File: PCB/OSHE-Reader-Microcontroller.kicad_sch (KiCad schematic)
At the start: 1 part

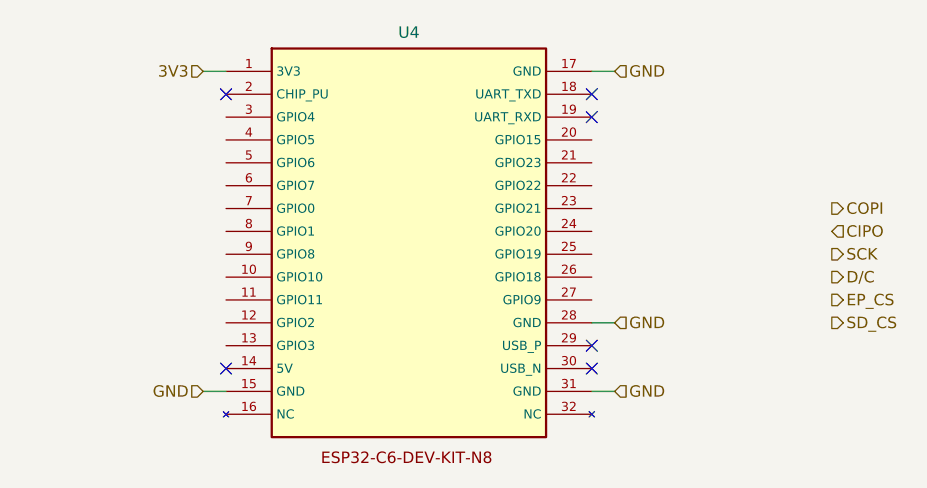
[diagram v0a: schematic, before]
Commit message: HOPEFULLY GOOD FOR EVER (good for first semester) :)
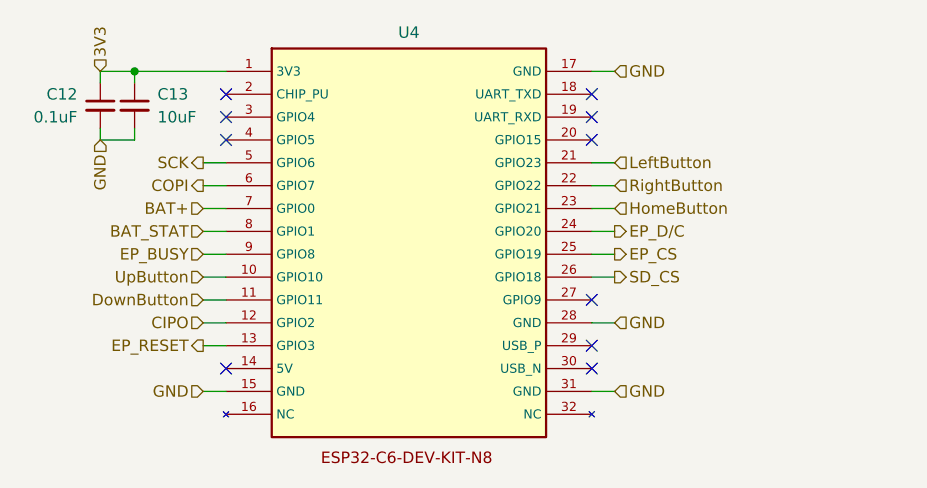
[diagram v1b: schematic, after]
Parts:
- added C12: 0.1uF, symbol Device:C_Small
- added C13: 10uF, symbol Device:C_Small
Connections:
- net 3V3: now also C12.1, C13.1
- net CIPO: now also U4.12 (GPIO2)
- net COPI: now also U4.6 (GPIO7)
- net EP_CS: now also U4.25 (GPIO19)
- net GND: now also C12.2, C13.2
- net SCK: now also U4.5 (GPIO6)
- net SD_CS: now also U4.26 (GPIO18)
- net UpButton: now reaches U4.10 (GPIO10)
- net DownButton: now reaches U4.11 (GPIO11)
- net EP_RESET: now reaches U4.13 (GPIO3)
- net LeftButton: now reaches U4.21 (GPIO23)
- net RightButton: now reaches U4.22 (GPIO22)
- net HomeButton: now reaches U4.23 (GPIO21)
- net EP_D/C: now reaches U4.24 (GPIO20)
- net BAT+: now reaches U4.7 (GPIO0)
- net BAT_STAT: now reaches U4.8 (GPIO1)
- net EP_BUSY: now reaches U4.9 (GPIO8)
- no-connect marks 6 -> 10

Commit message: small
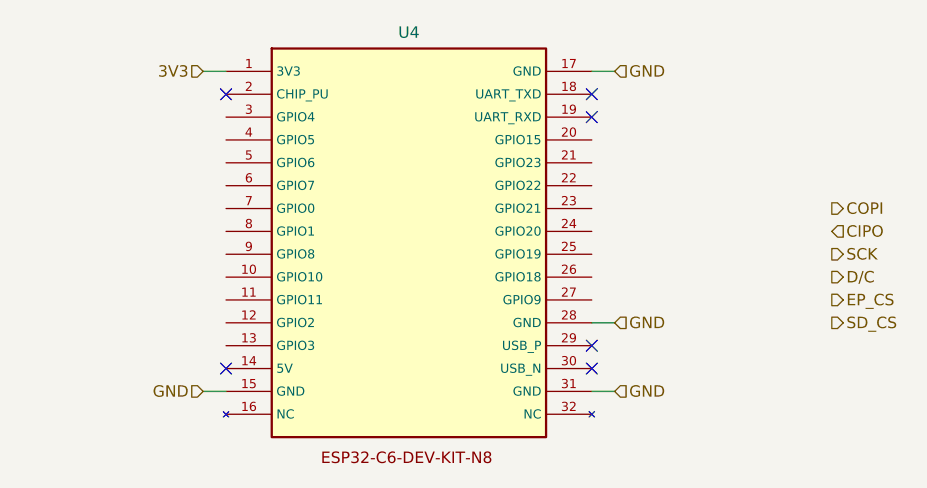
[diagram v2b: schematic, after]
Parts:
- removed C12: 0.1uF, symbol Device:C_Small
- removed C13: 10uF, symbol Device:C_Small
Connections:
- net CIPO: no longer U4.12 (GPIO2)
- net COPI: no longer U4.6 (GPIO7)
- net EP_CS: no longer U4.25 (GPIO19)
- net SCK: no longer U4.5 (GPIO6)
- net SD_CS: no longer U4.26 (GPIO18)
- net BAT+: no longer names the net of U4.7 (GPIO0)
- net BAT_STAT: no longer names the net of U4.8 (GPIO1)
- net DownButton: no longer names the net of U4.11 (GPIO11)
- net EP_BUSY: no longer names the net of U4.9 (GPIO8)
- net EP_D/C: no longer names the net of U4.24 (GPIO20)
- net EP_RESET: no longer names the net of U4.13 (GPIO3)
- net HomeButton: no longer names the net of U4.23 (GPIO21)
- net LeftButton: no longer names the net of U4.21 (GPIO23)
- net RightButton: no longer names the net of U4.22 (GPIO22)
- net UpButton: no longer names the net of U4.10 (GPIO10)
- no-connect marks 10 -> 6
